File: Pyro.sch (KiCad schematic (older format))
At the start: 14 parts, among them P6 TERM_BLOCK_2.54MM_2POS, P7 TERM_BLOCK_2.54MM_8POS, Q1 DMN2041LSD, Q2 BSS138DW, Q3 DMN2041LSD, Q4 BSS138DW

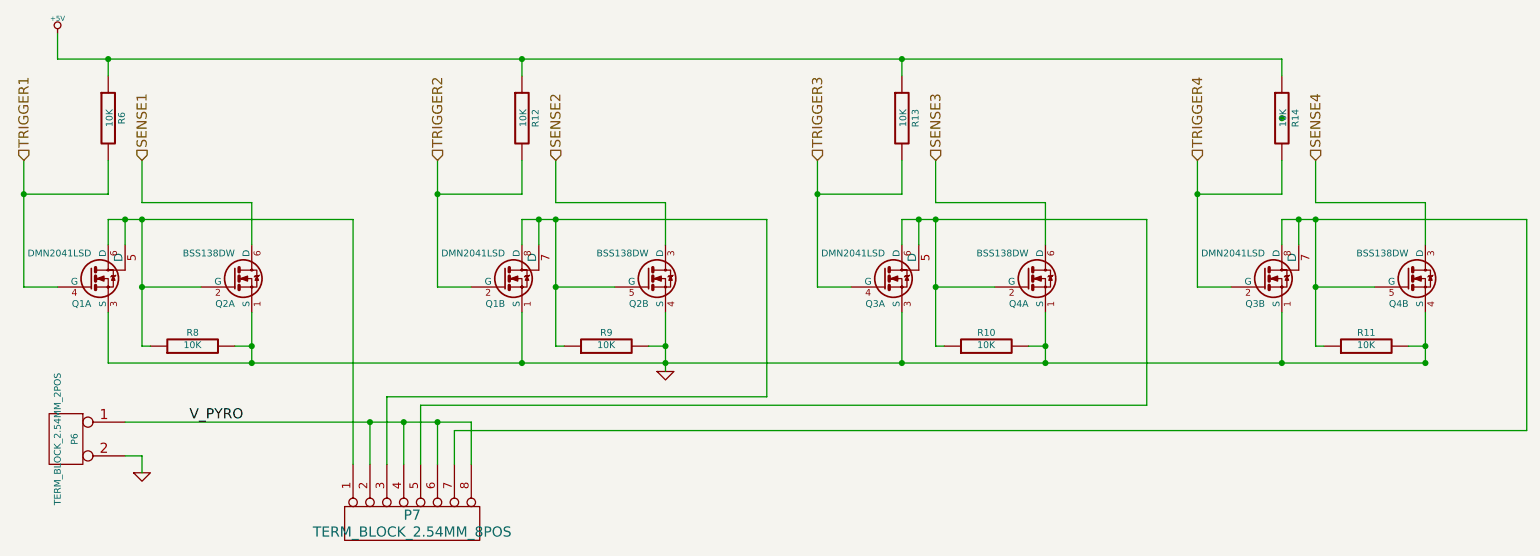
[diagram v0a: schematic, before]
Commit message: Improved schematic
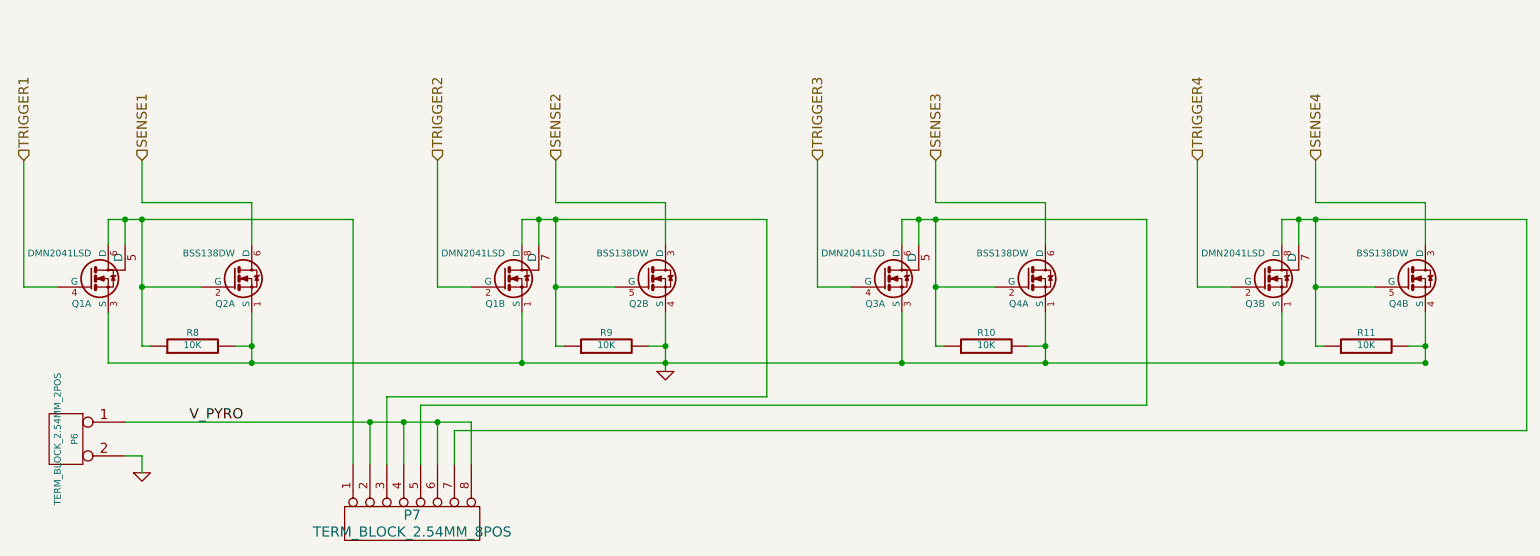
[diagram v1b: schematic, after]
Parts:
- removed R12, R13, R14, R6: 10K, ~, symbol R
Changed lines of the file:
@@
 Connection ~ 4500 2850
-Wire Wire Line
-	3150 1750 3150 2500
 Wire Wire Line
 	3150 2500 3350 2500
@@
 Wire Wire Line
 	9000 2950 9000 2650
-Wire Wire Line
-	900  1000 900  1150
-Wire Wire Line
-	900  1150 8150 1150
-$Comp
-L R R6
-U 1 1 548277E3
-P 1200 1500
-F 0 "R6" V 1280 1500 40  0000 C CNN
-F 1 "10K" V 1207 1501 40  0000 C CNN
-F 2 "~" V 1130 1500 30  0000 C CNN
-F 3 "~" H 1200 1500 30  0000 C CNN
-	1    1200 1500
-	1    0    0    -1
-$EndComp
-Wire Wire Line
-	1200 1750 1200 1950
-Wire Wire Line
-	1200 1950 700  1950
-Connection ~ 700  1950
-Wire Wire Line
-	1200 1250 1200 1150
-Connection ~ 1200 1150
-$Comp
-L R R12
-U 1 1 548278C1
-P 3650 1500
-F 0 "R12" V 3730 1500 40  0000 C CNN
-F 1 "10K" V 3657 1501 40  0000 C CNN
-F 2 "~" V 3580 1500 30  0000 C CNN
-F 3 "~" H 3650 1500 30  0000 C CNN
-	1    3650 1500
-	1    0    0    -1
-$EndComp
-$Comp
-L R R14
-U 1 1 548278CC
-P 8150 1500
-F 0 "R14" V 8230 1500 40  0000 C CNN
-F 1 "10K" V 8157 1501 40  0000 C CNN
-F 2 "~" V 8080 1500 30  0000 C CNN
-F 3 "~" H 8150 1500 30  0000 C CNN
-	1    8150 1500
-	1    0    0    -1
-$EndComp
-$Comp
-L R R13
-U 1 1 548278D2
-P 5900 1500
-F 0 "R13" V 5980 1500 40  0000 C CNN
-F 1 "10K" V 5907 1501 40  0000 C CNN
-F 2 "~" V 5830 1500 30  0000 C CNN
-F 3 "~" H 5900 1500 30  0000 C CNN
-	1    5900 1500
-	1    0    0    -1
-$EndComp
-Wire Wire Line
-	8150 1150 8150 1250
-Wire Wire Line
-	8150 1750 8150 1950
-Wire Wire Line
-	8150 1950 7650 1950
-Connection ~ 7650 1950
-Wire Wire Line
-	5900 1150 5900 1250
-Connection ~ 5900 1150
-Wire Wire Line
-	5900 1750 5900 1950
-Wire Wire Line
-	5900 1950 5400 1950
-Connection ~ 5400 1950
-Wire Wire Line
-	3650 1750 3650 1950
-Wire Wire Line
-	3650 1950 3150 1950
-Connection ~ 3150 1950
-Wire Wire Line
-	3650 1250 3650 1150
-Connection ~ 3650 1150
-$Comp
-L +5V #PWR30
-U 1 1 5482887D
-P 900 1000
-F 0 "#PWR30" H 900 1090 20  0001 C CNN
-F 1 "+5V" H 900 1090 30  0000 C CNN
-F 2 "" H 900 1000 60  0000 C CNN
-F 3 "" H 900 1000 60  0000 C CNN
-	1    900  1000
-	1    0    0    -1
-$EndComp
 $Comp
 L TERM_BLOCK_2.54MM_2POS P6
@@
 	0    -1   1    0
 $EndComp
-Connection ~ 8150 1500
 $Comp
 L DMN2041LSD Q1
@@
 	1    0    0    -1
 $EndComp
+Wire Wire Line
+	3150 1750 3150 2500
 $EndSCHEMATC
